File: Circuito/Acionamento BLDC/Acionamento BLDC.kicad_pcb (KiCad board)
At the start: 2 copper layers, 146.1 x 113 mm, 37 parts, among them J1 42V, J2 Motor, J3 Hall, J4 Potenciômetro, Q1 FDH50N50, Q2 FDH50N50, Q3 FDH50N50, Q4 FDH50N50, Q5 FDH50N50, Q6 FDH50N50, U1 MC33035

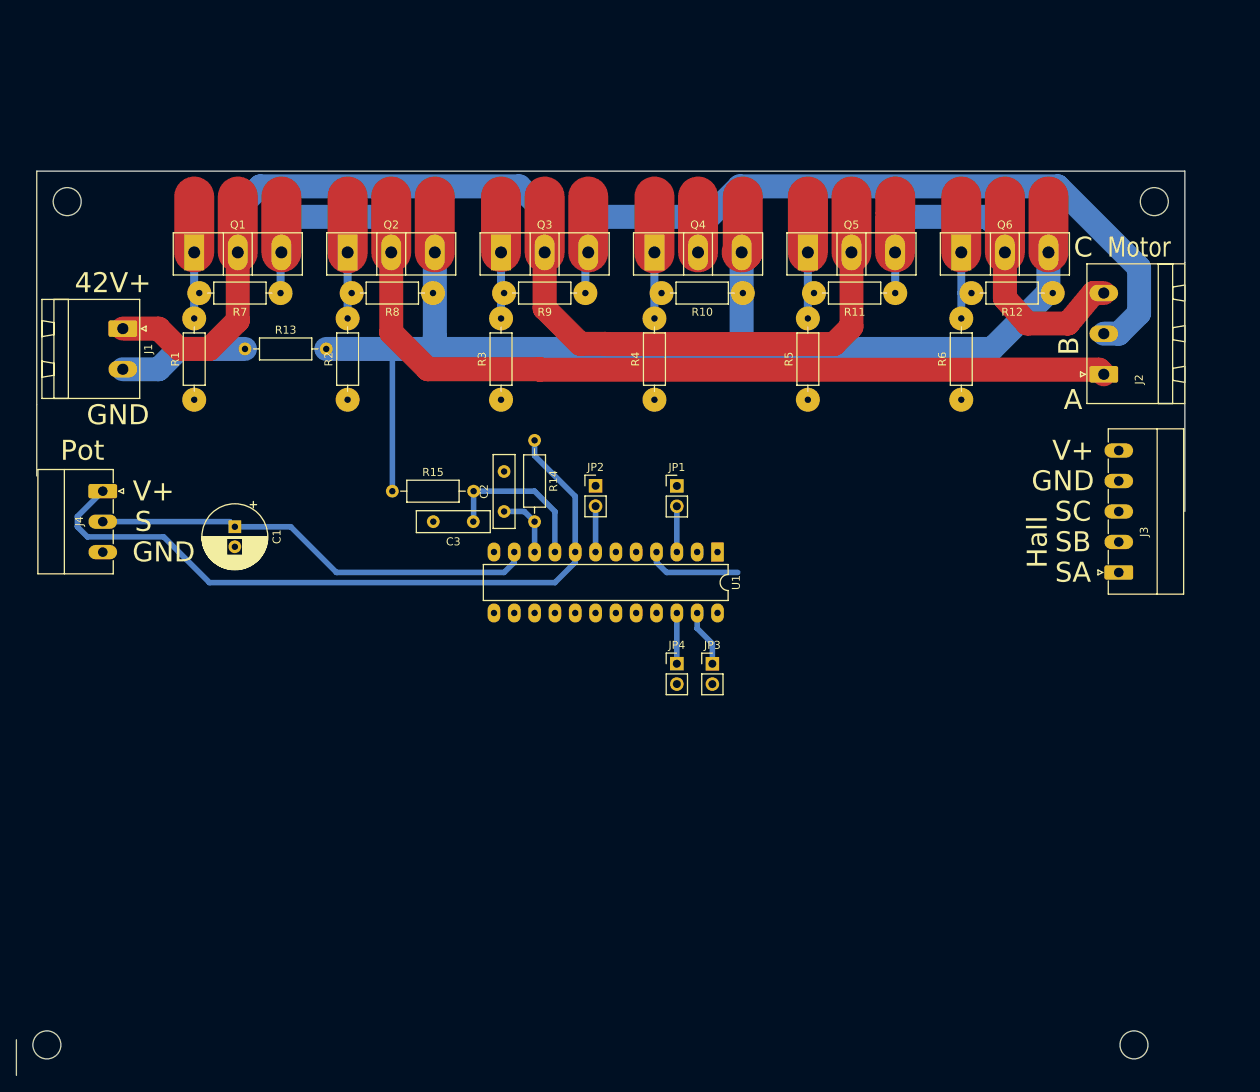
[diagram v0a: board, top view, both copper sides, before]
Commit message: Versão 2023
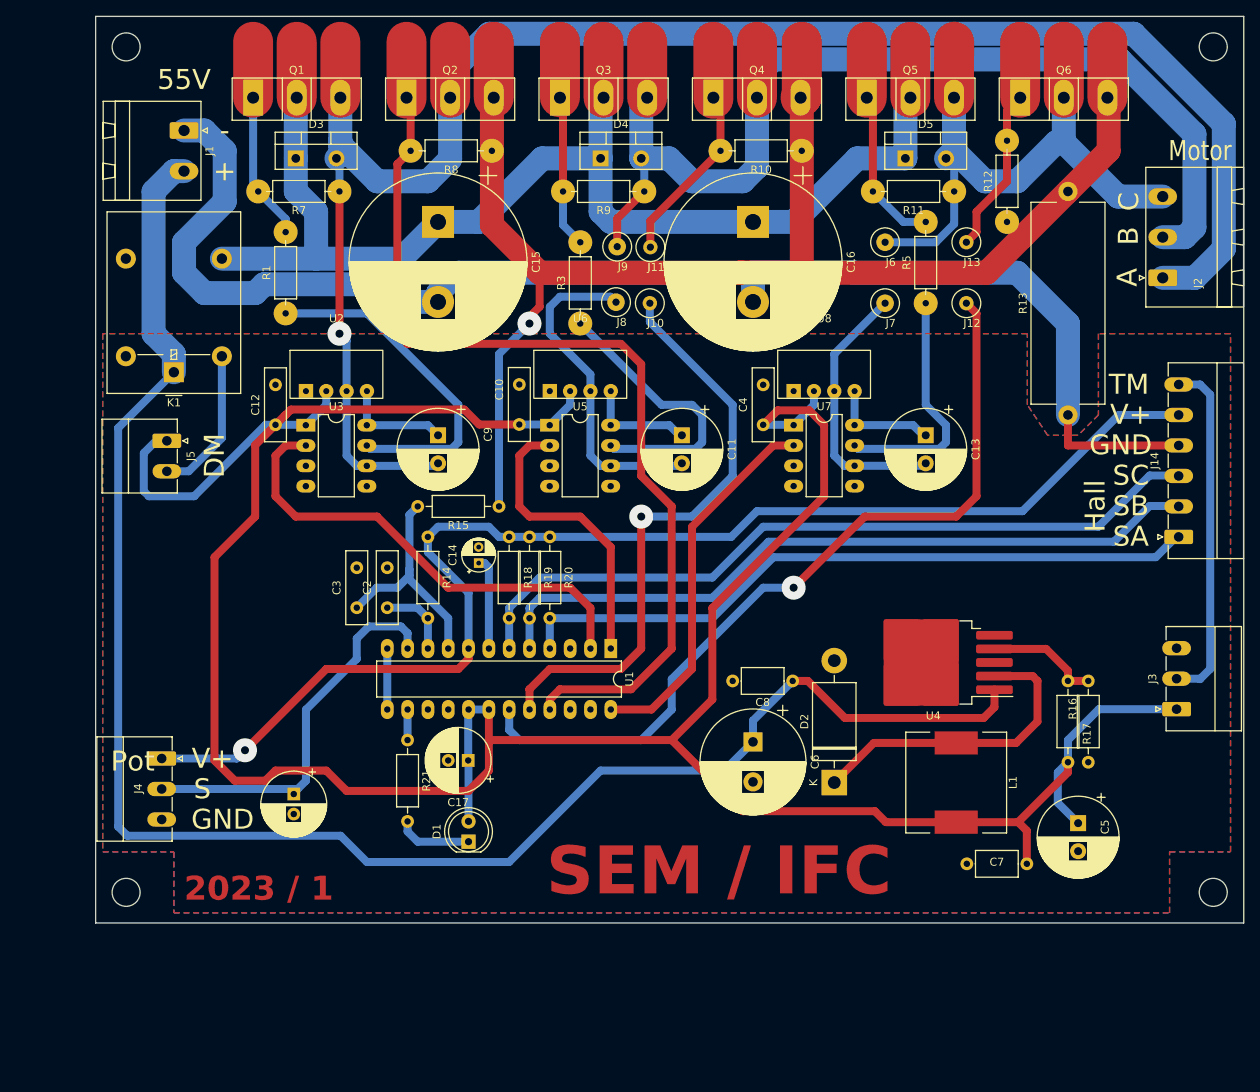
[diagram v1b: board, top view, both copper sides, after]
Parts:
- removed JP1, JP2, JP3, JP4: Jumper_2_Open, Connector_PinHeader_2.54mm:PinHeader_1x02_P2.54mm_Vertical
- removed R2, R4, R6: R, Resistor_THT:R_Axial_DIN0207_L6.3mm_D2.5mm_P10.16mm_Horizontal
- added C10: C, Capacitor_THT:C_Disc_D9.0mm_W2.5mm_P5.00mm, F.Cu at (119.4, 82.5)
- added C11: 470u 16V, Capacitor_THT:CP_Radial_D10.0mm_P3.50mm, F.Cu at (139.7, 83.8)
- added C12: C, Capacitor_THT:C_Disc_D9.0mm_W2.5mm_P5.00mm, F.Cu at (88.9, 82.5)
- added C13: 470u 16V, Capacitor_THT:CP_Radial_D10.0mm_P3.50mm, F.Cu at (170.2, 83.8)
- added C14: 2,2u, Capacitor_THT:CP_Radial_D4.0mm_P2.00mm, F.Cu at (114.3, 99.8)
- added C15: 470u 100V, Capacitor_THT:CP_Radial_D22.0mm_P10.00mm_SnapIn, F.Cu at (109.2, 57.1)
- added C16: 470u 100V, Capacitor_THT:CP_Radial_D22.0mm_P10.00mm_SnapIn, F.Cu at (148.6, 57.1)
- added C17: 100u 16V, Capacitor_THT:CP_Radial_D8.0mm_P2.50mm, F.Cu at (113.0, 124.5)
- added C4: C, Capacitor_THT:C_Disc_D9.0mm_W2.5mm_P5.00mm, F.Cu at (149.9, 82.5)
- added C5: 470u 16V, Capacitor_THT:CP_Radial_D10.0mm_P3.50mm, F.Cu at (189.2, 132.3)
- added C6: 470u 63V, Capacitor_THT:CP_Radial_D13.0mm_P5.00mm, F.Cu at (148.6, 122.1)
- added C7: 100n, Capacitor_THT:C_Axial_L5.1mm_D3.1mm_P7.50mm_Horizontal, F.Cu at (182.8, 137.4)
- added C8: 100n, Capacitor_THT:C_Axial_L5.1mm_D3.1mm_P7.50mm_Horizontal, F.Cu at (153.6, 114.5)
- added C9: 470u 16V, Capacitor_THT:CP_Radial_D10.0mm_P3.50mm, F.Cu at (109.2, 83.8)
- added D1: LED, LED_THT:LED_D5.0mm, F.Cu at (113.0, 134.6)
- added D2: 1N5822, Diode_THT:D_DO-201AD_P15.24mm_Horizontal, F.Cu at (158.8, 127.2)
- added D3: Verificar, Package_TO_SOT_THT:TO-220-2_Vertical, F.Cu at (91.4, 49.2)
- added D4: Verificar, Package_TO_SOT_THT:TO-220-2_Vertical, F.Cu at (129.5, 49.2)
- added D5: Verificar, Package_TO_SOT_THT:TO-220-2_Vertical, F.Cu at (167.6, 49.2)
- added J10: ~, TestPoint:TestPoint_Loop_D3.50mm_Drill0.9mm_Beaded, F.Cu at (135.7, 67.3)
- added J11: ~, TestPoint:TestPoint_Loop_D3.50mm_Drill0.9mm_Beaded, F.Cu at (135.8, 60.3)
- added J12: ~, TestPoint:TestPoint_Loop_D3.50mm_Drill0.9mm_Beaded, F.Cu at (175.3, 67.3)
- added J13: ~, TestPoint:TestPoint_Loop_D3.50mm_Drill0.9mm_Beaded, F.Cu at (175.3, 59.7)
- added J14: Sensores, Connector_Phoenix_MC:PhoenixContact_MC_1,5_6-G-3.81_1x06_P3.81mm_Horizontal, F.Cu at (201.8, 96.5)
- added J5: DM, Connector_Phoenix_MC:PhoenixContact_MC_1,5_2-G-3.81_1x02_P3.81mm_Horizontal, F.Cu at (75.3, 84.5)
- added J6: ~, TestPoint:TestPoint_Loop_D3.50mm_Drill0.9mm_Beaded, F.Cu at (165.1, 59.7)
- added J7: ~, TestPoint:TestPoint_Loop_D3.50mm_Drill0.9mm_Beaded, F.Cu at (165.1, 67.3)
- added J8: ~, TestPoint:TestPoint_Loop_D3.50mm_Drill0.9mm_Beaded, F.Cu at (131.5, 67.2)
- added J9: ~, TestPoint:TestPoint_Loop_D3.50mm_Drill0.9mm_Beaded, F.Cu at (131.6, 60.2)
- added K1: G5LE-1, Relay_THT:Relay_SPDT_Omron-G5LE-1, F.Cu at (76.2, 75.9)
- added L1: 100u, Inductor_SMD:L_12x12mm_H6mm, F.Cu at (174.0, 127.2)
- added R16: 9,1K, Resistor_THT:R_Axial_DIN0207_L6.3mm_D2.5mm_P10.16mm_Horizontal, F.Cu at (188.0, 114.5)
- added R17: 1K, Resistor_THT:R_Axial_DIN0207_L6.3mm_D2.5mm_P10.16mm_Horizontal, F.Cu at (190.5, 124.7)
- added R18: 1K, Resistor_THT:R_Axial_DIN0207_L6.3mm_D2.5mm_P10.16mm_Horizontal, F.Cu at (118.1, 96.5)
- added R19: 1K, Resistor_THT:R_Axial_DIN0207_L6.3mm_D2.5mm_P10.16mm_Horizontal, F.Cu at (120.7, 96.5)
- added R20: 1K, Resistor_THT:R_Axial_DIN0207_L6.3mm_D2.5mm_P10.16mm_Horizontal, F.Cu at (123.2, 96.5)
- added R21: 1K, Resistor_THT:R_Axial_DIN0207_L6.3mm_D2.5mm_P10.16mm_Horizontal, F.Cu at (105.4, 121.9)
- added U2: B1212s-1W, B1212s-1W:B1212s-1W, F.Cu at (96.5, 76.2)
- added U3: IR2118, Package_DIP:DIP-8_W7.62mm_LongPads, F.Cu at (92.7, 82.6)
- added U4: LM2596S-ADJ, Package_TO_SOT_SMD:TO-263-5_TabPin3, F.Cu at (171.1, 112.2)
- added U5: IR2118, Package_DIP:DIP-8_W7.62mm_LongPads, F.Cu at (123.2, 82.6)
- added U6: B1212s-1W, B1212s-1W:B1212s-1W, F.Cu at (127.0, 76.2)
- added U7: IR2118, Package_DIP:DIP-8_W7.62mm_LongPads, F.Cu at (153.7, 82.5)
- added U8: B1212s-1W, B1212s-1W:B1212s-1W, F.Cu at (157.5, 76.2)
- C2: value C -> 100n
- J1: value 42V -> 55V
- J3: value Hall -> Telemetria; footprint Connector_Phoenix_MC:PhoenixContact_MC_1,5_5-G-3.81_1x05_P3.81mm_Horizontal -> Connector_Phoenix_MC:PhoenixContact_MC_1,5_3-G-3.81_1x03_P3.81mm_Horizontal
- R1, R3, R5: value R -> 10
- R10, R11, R12, R7, R8, R9: value R -> 100K
- R13: value R -> 0,01; footprint Resistor_THT:R_Axial_DIN0207_L6.3mm_D2.5mm_P10.16mm_Horizontal -> Resistor_THT:R_Axial_Power_L25.0mm_W9.0mm_P27.94mm
- R14: value R -> 1K
- moved R13 103.2 mm to (188.0, 81.3), turned to 90 degrees
- moved C1 34.2 mm to (91.2, 128.7)
- moved J4 34.2 mm to (74.7, 124.2)
- moved J1 25.9 mm to (77.5, 45.7)
- moved H2 21.5 mm to (206.1, 140.9)
- moved H3 21.5 mm to (70.2, 140.9)
- moved H4 20.7 mm to (206.1, 35.3)
- moved Q4 20.7 mm to (143.6, 41.6)
- moved Q6 20.7 mm to (182.0, 41.6)
- moved H1 20.7 mm to (70.2, 35.3)
- moved Q1 20.7 mm to (86.1, 41.6)
- moved Q2 20.7 mm to (105.3, 41.6)
- moved Q3 20.7 mm to (124.5, 41.6)
- moved Q5 20.7 mm to (162.8, 41.6)
- moved R10 19.2 mm to (154.7, 48.3)
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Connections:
- J1 pad 1: /V42+ -> GND
- J1 pad 2: GND -> /V55+
- J3 pad 1: /SA -> +12V
- J3 pad 2: /SB -> /TempMot
- J3 pad 3: /SC -> GND
- Q1 pad 2: /V42+ -> Net-(D3-K)
- Q2 pad 1: Net-(Q2-Pad1) -> /AL
- Q3 pad 2: /V42+ -> Net-(D3-K)
- Q5 pad 2: /V42+ -> Net-(D3-K)
- R8 pad 2: Net-(Q2-Pad1) -> /AL
- U1 pad 14: unconnected-(U1-Pad14) -> Net-(U1-Fault)
- U1 pad 17: unconnected-(U1-Pad17) -> +12V
- U1 pad 18: unconnected-(U1-Pad18) -> +12V
- U1 pad 22: Net-(JP4-Pad1) -> GND
- U1 pad 23: Net-(JP3-Pad1) -> GND
- U1 pad 3: Net-(U1-Pad3) -> GND
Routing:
- net +12V: track 0.00 -> 365.1 mm
- net /V55+: track 0.00 -> 215.2 mm
- net Net-(D3-K): track 0.00 -> 160.5 mm
- net GND: track 16.3 -> 174.0 mm
- net /V42+: track 154.2 -> 0.00 mm
- net /AL: track 0.00 -> 125.8 mm
- net /CL: track 0.00 -> 101.0 mm, vias 0 -> 1
- net /SC: track 0.00 -> 95.4 mm
- net /SB: track 0.00 -> 91.2 mm
- net /FaseA: track 141.6 -> 228.6 mm, vias 0 -> 1
- net /BL: track 0.00 -> 74.5 mm, vias 0 -> 1
- net /SA: track 12.0 -> 86.4 mm
- net +6V: track 89.3 -> 162.1 mm, vias 0 -> 1
- net /DAH: track 0.00 -> 59.6 mm
- net /DCH: track 0.00 -> 46.9 mm
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- added copper zone on B.Cu, net GND
- added copper zone on F.Cu, net GND
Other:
- board size 146.1 x 113 mm -> 143.5 x 113.3 mm
- board text added: "+"
- board text added: "-"
- board text added: "2023 / 1"
- board text added: "55V"
- board text added: "DM"
- board text added: "SEM / IFC"
- board text added: "TM"
- board text removed: "42V+"
